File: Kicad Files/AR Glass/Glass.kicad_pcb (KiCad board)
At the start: 2 copper layers, 149.4 x 56.7 mm, 16 parts, among them U1 Pico, U2 OLED Driver, U3 OLED Driver 2, U4 Camera

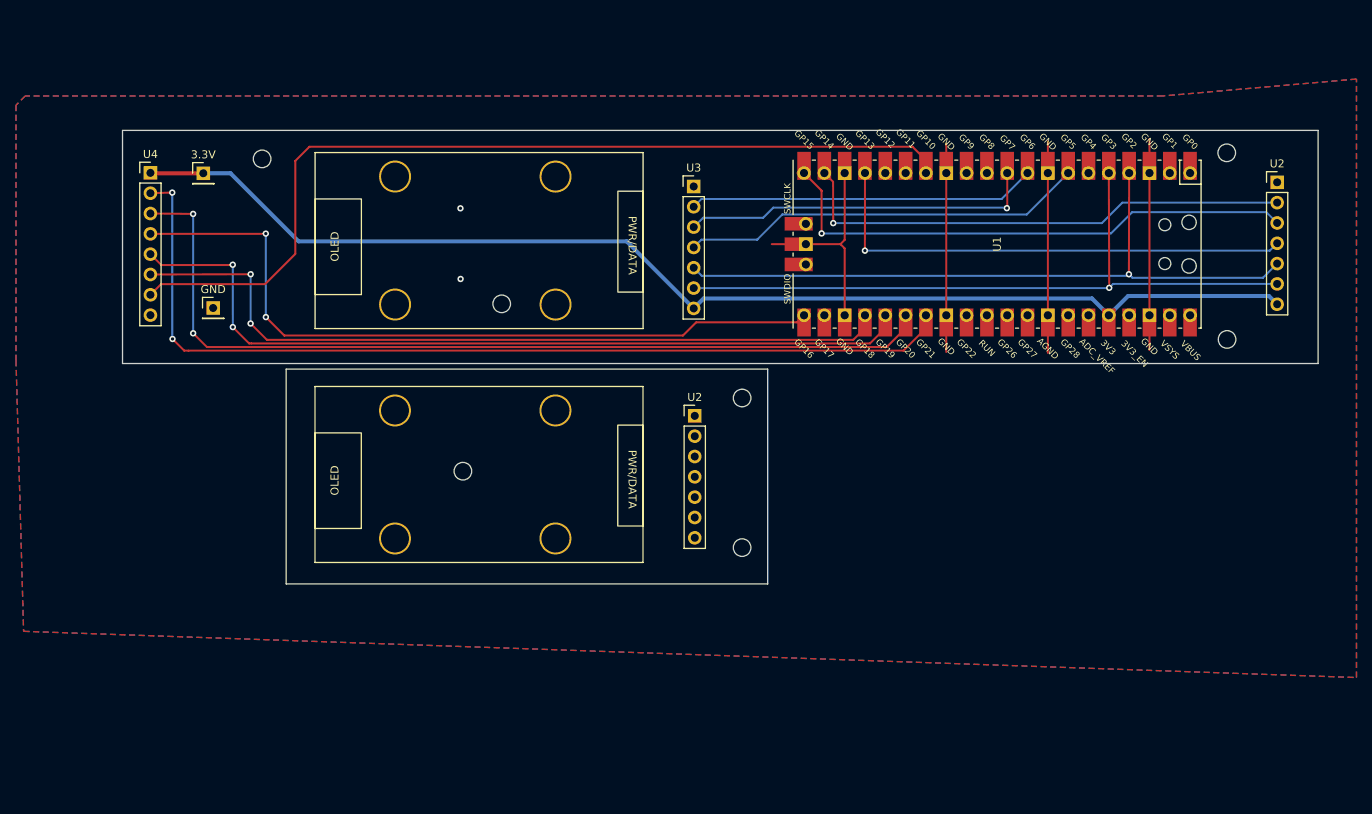
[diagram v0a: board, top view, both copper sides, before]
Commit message: AR revised
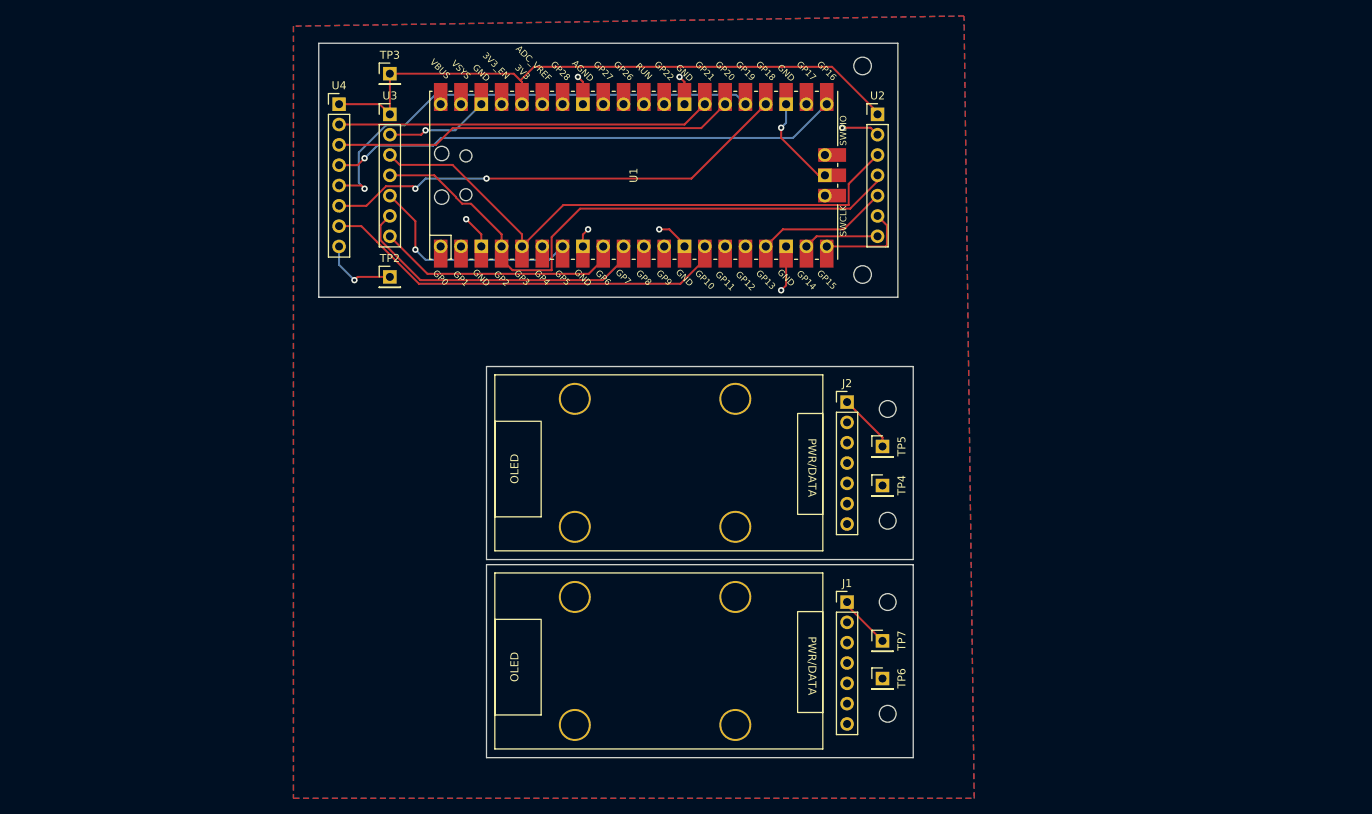
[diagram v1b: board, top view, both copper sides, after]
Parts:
- removed 3.3V, GND: TestPoint, Connector_PinHeader_2.54mm:PinHeader_1x01_P2.54mm_Vertical
- removed the REF** at (136.3, 56.7)
- removed the REF** at (219.6, 67.1)
- removed the REF** at (158.9, 93.1)
- removed the REF** at (128.9, 62.6)
- removed the REF** at (158.9, 74.4)
- removed the REF** at (99.0, 44.5)
- removed the REF** at (136.3, 85.9)
- removed the REF** at (124.0, 83.6)
- removed the REF** at (219.5, 43.8)
- removed the U2 at (225.8, 47.5)
- removed the U2 at (153.0, 76.7)
- added J1: Conn_01x07_Pin, Connector_PinHeader_2.54mm:PinHeader_1x07_P2.54mm_Vertical, F.Cu at (172.1, 99.9)
- added J2: Conn_01x07_Pin, Connector_PinHeader_2.54mm:PinHeader_1x07_P2.54mm_Vertical, F.Cu at (172.1, 74.9)
- added REF**: MountingHole_2.1mm, MountingHole:MountingHole_2.1mm, F.Cu at (177.2, 99.9)
- added REF**: MountingHole_2.2mm_M2, MountingHole:MountingHole_2.2mm_M2, F.Cu at (174.0, 32.9)
- added REF**: MountingHole_2.1mm, MountingHole:MountingHole_2.1mm, F.Cu at (177.2, 75.8)
- added REF**: OLED Driver, MCU_RaspberryPi_and_Boards:OLED Driver, F.Cu at (158.8, 109.2)
- added REF**: MountingHole_2.1mm, MountingHole:MountingHole_2.1mm, F.Cu at (177.2, 113.9)
- added REF**: MountingHole_2.1mm, MountingHole:MountingHole_2.1mm, F.Cu at (177.2, 89.8)
- added REF**: OLED Driver, MCU_RaspberryPi_and_Boards:OLED Driver, F.Cu at (158.8, 84.5)
- added REF**: MountingHole_2.2mm_M2, MountingHole:MountingHole_2.2mm_M2, F.Cu at (174.0, 59.0)
- added TP2: TestPoint, Connector_PinHeader_2.54mm:PinHeader_1x01_P2.54mm_Vertical, F.Cu at (114.9, 59.3)
- added TP3: TestPoint, Connector_PinHeader_2.54mm:PinHeader_1x01_P2.54mm_Vertical, F.Cu at (114.9, 33.9)
- added TP4: TestPoint, Connector_PinHeader_2.54mm:PinHeader_1x01_P2.54mm_Vertical, F.Cu at (176.5, 85.4)
- added TP5: TestPoint, Connector_PinHeader_2.54mm:PinHeader_1x01_P2.54mm_Vertical, F.Cu at (176.5, 80.5)
- added TP6: TestPoint, Connector_PinHeader_2.54mm:PinHeader_1x01_P2.54mm_Vertical, F.Cu at (176.5, 109.5)
- added TP7: TestPoint, Connector_PinHeader_2.54mm:PinHeader_1x01_P2.54mm_Vertical, F.Cu at (176.5, 104.8)
- added U2: OLED Driver, Connector_PinHeader_2.54mm:PinHeader_1x07_P2.54mm_Vertical, F.Cu at (175.9, 39.0)
- U3: value OLED Driver 2 -> OLED Driver
- moved U1 46.2 mm to (145.4, 46.6), turned to 90 degrees
- moved U3 39.0 mm to (114.9, 39.0)
- moved U4 25.1 mm to (108.6, 37.7)
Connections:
- U1 pad 10: /GP7 -> GP7
- U1 pad 17: /GP13 -> GP13
- U1 pad 19: /GP14 -> GP14
- U1 pad 20: /GP15 -> GP15
- U1 pad 36: +3.3V -> 3.3V
- U1 pad 4: /GP2 -> GP2
- U1 pad 5: /GP3 -> GP3
- U1 pad 7: /GP5 -> GP5
- U1 pad 9: /GP6 -> GP6
- U3 pad 1: GND -> 3.3V
- U3 pad 2: /GP6 -> GND
- U3 pad 3: /GP7 -> GP3
- U3 pad 4: /GP5 -> GP2
- U3 pad 5: /GP2 -> GP5
- U3 pad 6: /GP3 -> GP7
- U3 pad 7: +3.3V -> GP6
- U4 pad 1: +3.3V -> 3.3V
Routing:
- net +3.3V: track 150.7 -> 0.00 mm
- net 3.3V: track 0.00 -> 93.7 mm
- net /GP3: track 87.6 -> 0.00 mm, vias 1 -> 0
- net /GP2: track 87.0 -> 0.00 mm, vias 1 -> 0
- net GP2: track 0.00 -> 75.5 mm
- net GP3: track 0.00 -> 72.9 mm
- net /GP21: track 118.7 -> 46.8 mm, vias 2 -> 0
- net /GP15: track 68.0 -> 0.00 mm, vias 1 -> 0
- net /GP14: track 63.3 -> 0.00 mm, vias 1 -> 0
- net /GP20: track 112.7 -> 50.4 mm, vias 2 -> 0
- net /GP10: track 113.7 -> 51.6 mm
- net /GP13: track 61.6 -> 0.00 mm, vias 1 -> 0
- net /GP5: track 50.7 -> 0.00 mm
- net /GP7: track 44.7 -> 0.00 mm, vias 1 -> 0
- net /GP19: track 103.7 -> 60.0 mm, vias 2 -> 1
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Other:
- board size 149.4 x 56.7 mm -> 74.3 x 89.3 mm
